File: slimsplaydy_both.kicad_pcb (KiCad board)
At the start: 2 copper layers, 139.6 x 179.5 mm, 84 parts

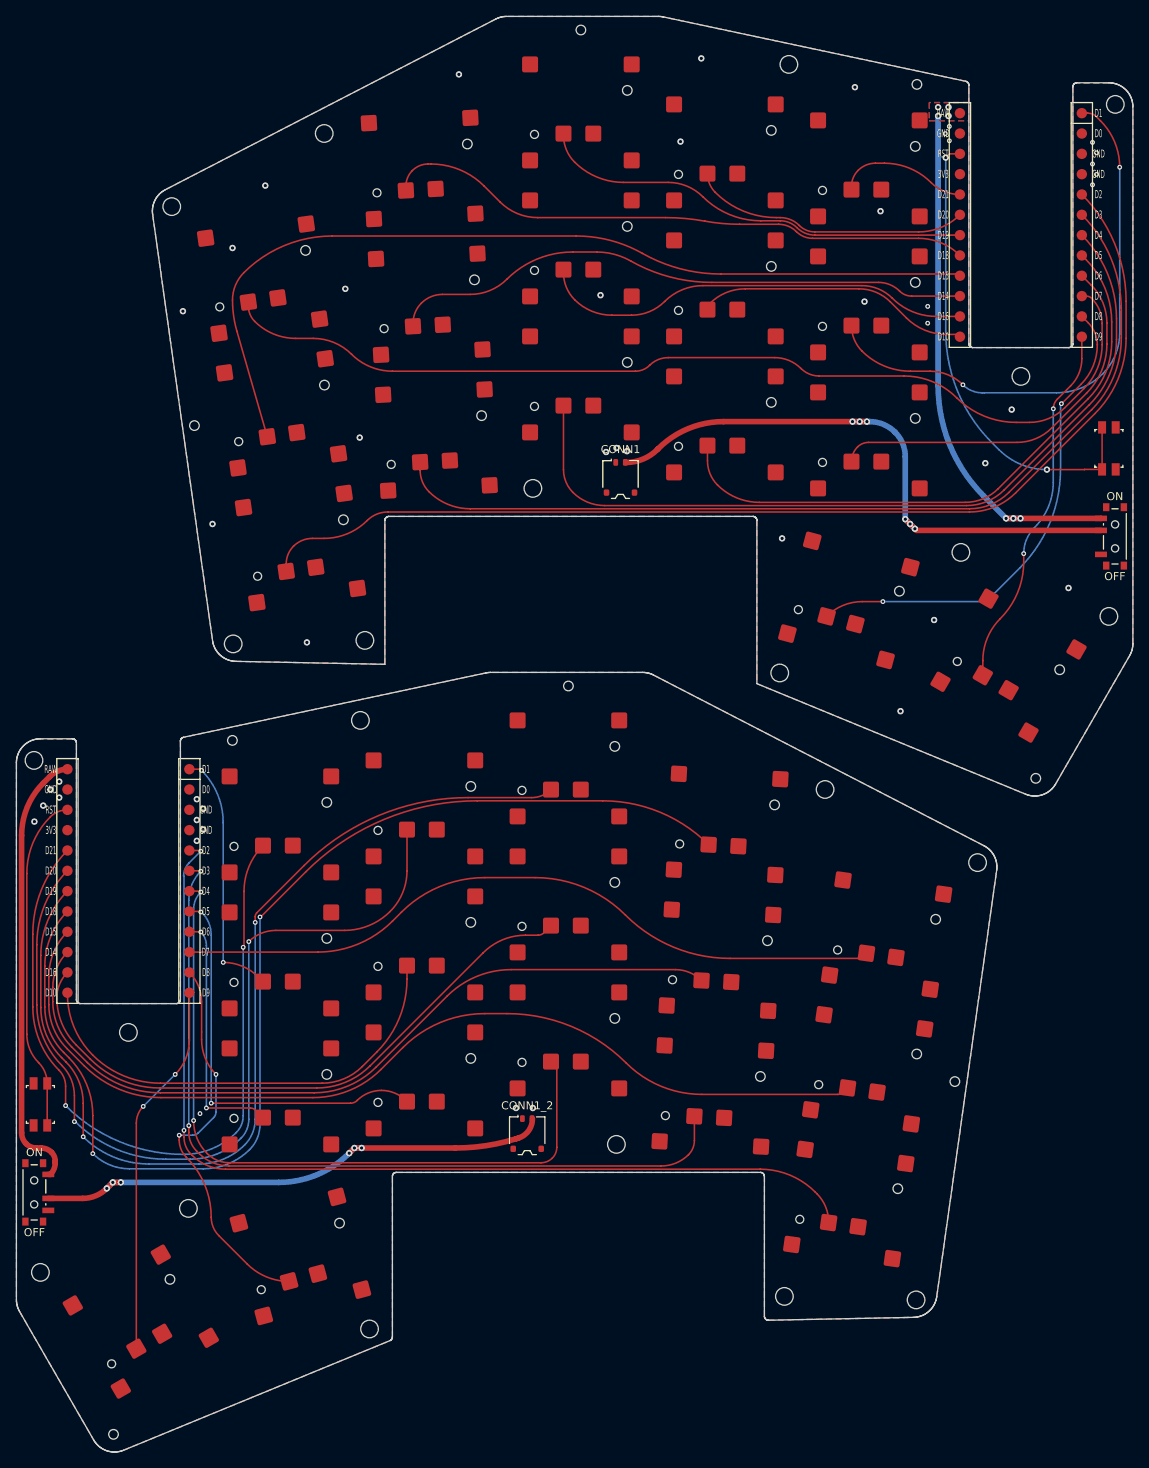
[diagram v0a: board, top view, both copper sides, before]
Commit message: Complete panel.
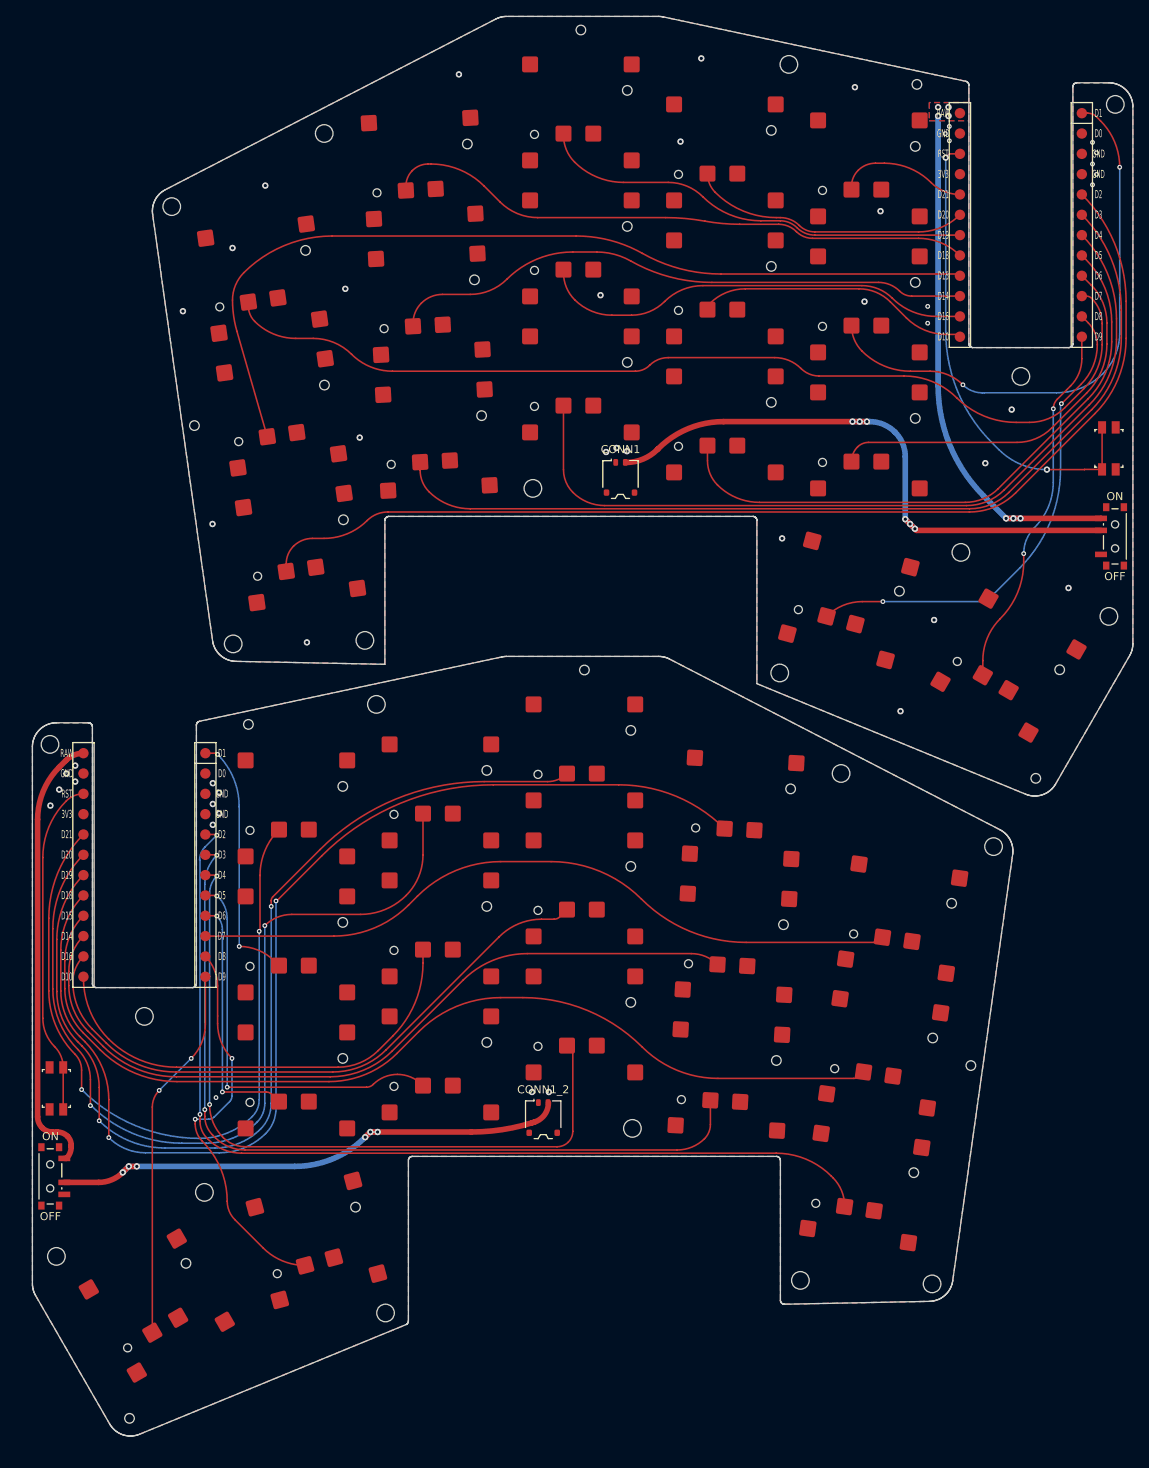
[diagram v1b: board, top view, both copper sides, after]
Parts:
- removed the ? at (90.0, 164.5)
- removed the ? at (-19.0, 106.0)
- removed the ? at (108.0, 115.0)
- removed the ? at (-19.0, 151.0)
- removed the ? at (13.0, 173.5)
- added ?: , kikit:Tab, F.Cu at (-17.0, 104.0)
- added ?: , kikit:Tab, F.Cu at (110.0, 149.0)
- added ?: , kikit:Tab, F.Cu at (-17.0, 149.0)
- added ?: , kikit:Tab, F.Cu at (5.00, 181.5)
- added ?: , kikit:Tab, F.Cu at (110.0, 113.0)
- moved S13_2 2.83 mm to (18.0, 132.9)
- moved S14_2 2.83 mm to (18.0, 115.9)
- moved S15_2 2.83 mm to (18.0, 98.9)
- moved CONN1_2 2.83 mm to (48.8, 137.6)
- moved MAG1_2 2.83 mm to (44.0, 113.9)
- moved MCU1_2 2.83 mm to (-1.02, 104.7)
- moved MH10_2 2.83 mm to (60.0, 138.9)
- moved MH11_2 2.83 mm to (81.0, 157.9)
- moved MH12_2 2.83 mm to (97.4, 158.4)
- moved MH13_2 2.83 mm to (105.1, 103.7)
- moved MH14_2 2.83 mm to (86.1, 94.6)
- moved MH15_2 2.83 mm to (28.0, 85.9)
- moved MH1_2 2.83 mm to (-2.88, 175.2)
- moved MH2_2 2.83 mm to (102.3, 131.1)
- moved MH3_2 2.83 mm to (54.0, 81.6)
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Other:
- board size 139.6 x 179.5 mm -> 137.6 x 177.5 mm
